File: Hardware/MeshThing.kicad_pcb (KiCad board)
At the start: 2 copper layers, 25.7 x 27.8 mm, 31 parts, among them IC1 ATMEGA2564/1284/644RFR2, SW1 RST, U1 CONN_MICROSD, U2 XBEE, U3 XBEE

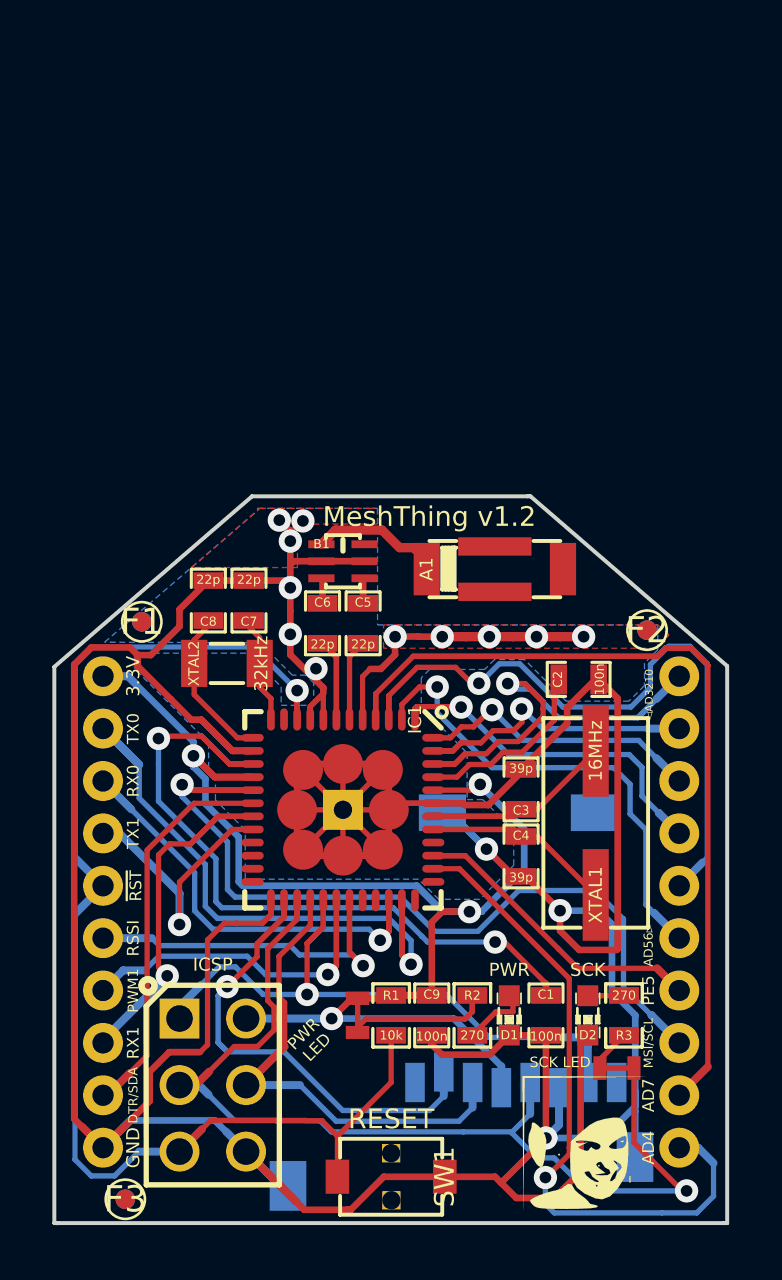
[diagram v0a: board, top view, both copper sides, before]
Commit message: Initial v2.0 commit.
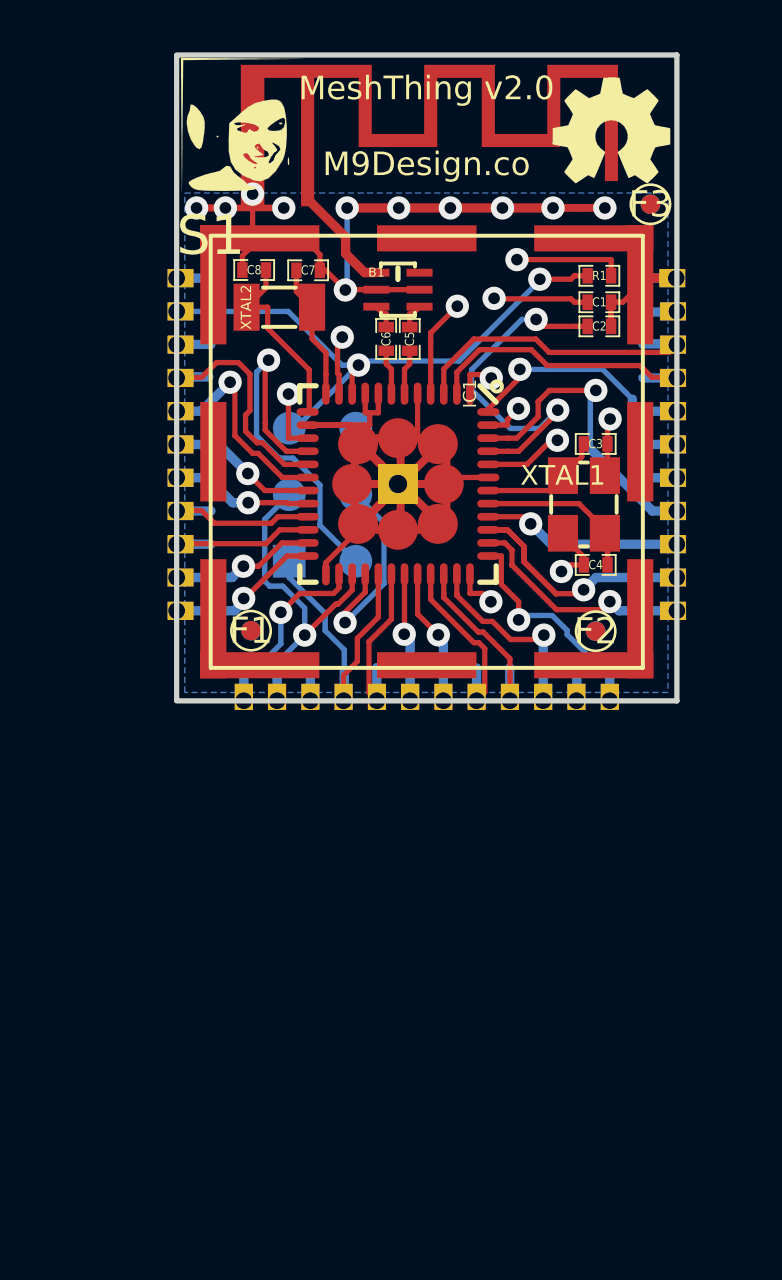
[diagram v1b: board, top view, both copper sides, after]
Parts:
- removed C9: 100n, _MT_SM0603_Capa
- removed D1, D2: LED, _MT_LED-0603
- removed the G*** at (155.9, 129.2)
- removed the G*** at (146.8, 108.7)
- removed H2: ICSP, _MT_pin_array_3x2
- removed R2, R3: 270, _MT_SM0603_Resistor
- removed SJ1, SJ2: SMTJPR, _MT_SMTJumper
- removed SW1: RST, _MT_TC007-TactileSwitch
- removed U1: CONN_MICROSD, _MT_microSD_3M_290805-A
- removed U2: XBEE, _MT_XBee_Board_STD_THPads
- removed U3: XBEE, _MT_XBee_Board_BackLablesOnly
- added G***: LOGO, _MT_OHW_LOGO:LOGO, F.Cu at (157.1, 90.5)
- added H1: ICSP, _MT_MC_Pretty:_MC_pin_pad_3x2, B.Cu at (146.0, 104.5)
- added P1: CONN34, _MT_MC_Pretty:_MC_CanFootprint-34Pin, F.Cu at (150.0, 100.0)
- added PrettyLady: PrettyLady, _MT_MC_Pretty:_MC_LOGO-PrettyLady, F.Cu at (142.9, 90.3)
- added S1: RFShield, _MT_MC_Pretty:_MT_MC_EMIShield-16.5x16.5, F.Cu at (150.0, 102.8)
- A1: value Antenna -> ANTENNA; footprint Johanson-2450AT42B100-PadsOnly -> _MT_MC_Pretty:_MT_IFA-2.4GHzPCBAntenna
- C1, C2, C5, C6, C7, C8: footprint _MT_SM0603_Capa -> SMD_Packages:SM0402_c
- C3, C4: value 39p -> 10p; footprint _MT_SM0603_Capa -> SMD_Packages:SM0402_c
- F1, F2, F3: value VAL** -> CONN_1; footprint _MT_Fiducial -> _MT_MC_Pretty:_MT_Fiducial
- R1: footprint _MT_SM0603_Resistor -> SMD_Packages:SM0402_r
- XTAL1: value 16MHz -> CRYSTAL_SMD-TSX3225; footprint _MT_CSM-3X-Crystal -> _MT_MC_Pretty:16MHz-3.2x2.5mm-TSX-3225
- XTAL2: footprint _MT_TF32D-32768-Crystal -> _MT_MC_Pretty:_MC_TF32D-32768-Crystal
- moved F3 43.0 mm to (158.5, 93.4)
- moved R1 29.3 mm to (156.6, 96.1), turned to 180 degrees
- moved C1 27.3 mm to (156.6, 97.1), turned to 0 degrees
- moved A1 16.9 mm to (150.0, 90.6)
- moved XTAL2 13.7 mm to (144.4, 97.3)
- moved C2 13.5 mm to (156.6, 98.0)
- moved C3 13.5 mm to (156.4, 102.5), turned to 0 degrees
- moved C7 12.8 mm to (145.5, 95.9), turned to 0 degrees
- moved C8 12.7 mm to (143.4, 95.9), turned to 180 degrees
- moved IC1 12.6 mm to (148.9, 104.0)
- moved XTAL1 12.2 mm to (156.0, 104.8), turned to 0 degrees
- moved C4 11.5 mm to (156.4, 107.1), turned to 180 degrees
- moved C6 11.1 mm to (148.4, 98.5)
- moved C5 11.0 mm to (149.3, 98.5)
- moved B1 10.6 mm to (148.9, 96.6)
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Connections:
- A1 pad 2: N-0000040 -> GND
- C3 pad 1: N-0000051 -> Net-(C3-Pad1)
- C4 pad 1: N-0000052 -> Net-(C4-Pad1)
- IC1 pad 11: N-0000049 -> PG1
- IC1 pad 21: N-0000048 -> PD4
- IC1 pad 22: N-0000047 -> PD5
- IC1 pad 23: N-0000046 -> PD6
- IC1 pad 24: N-0000044 -> PD7
- IC1 pad 32: N-0000021 -> PB6
- IC1 pad 33: N-0000045 -> PB7
- IC1 pad 36: N-0000022 -> PE2
- IC1 pad 37: N-0000020 -> PE3
- IC1 pad 40: N-0000050 -> PE7
- IC1 pad 41: N-0000052 -> Net-(C4-Pad1)
- IC1 pad 42: N-0000051 -> Net-(C3-Pad1)
- XTAL1 pad 1: N-0000052 -> Net-(C3-Pad1)
- XTAL1 pad 2: N-0000051 -> GND
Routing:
- net GND: track 226.8 -> 94.8 mm, vias 14 -> 13
- net PF7: track 45.6 -> 16.0 mm, vias 0 -> 1
- net Reset: track 49.1 -> 22.9 mm, vias 1 -> 2
- net SCK: track 39.6 -> 15.1 mm
- net SCL: track 33.1 -> 9.61 mm, vias 1 -> 0
- net PE4: track 25.6 -> 8.87 mm
- net TX0: track 24.8 -> 9.87 mm
- net PF6: track 26.3 -> 12.0 mm, vias 1 -> 0
- net PE7: track 0.00 -> 13.5 mm, vias 0 -> 1
- net MISO: track 25.1 -> 11.6 mm, vias 1 -> 0
- net Net-(C1-Pad1): track 28.0 -> 15.5 mm
- net PG1: track 0.00 -> 11.0 mm, vias 0 -> 1
- net N-0000052: track 10.7 -> 0.00 mm
- net N-0000051: track 10.7 -> 0.00 mm
- net RX0: track 17.3 -> 7.22 mm, vias 1 -> 0
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- added copper zone on Inner1.Cu, net +3.3V
- added copper zone on Inner2.Cu, net GND
- removed copper zone on F.Cu, net GND
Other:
- board size 25.7 x 27.8 mm -> 19.1 x 24.7 mm
- copper layers 2 -> 4
- net class 10mil added: clearance 0.2032, trace_width 0.254, via_dia 0.889, via_drill 0.635
- net class Default: trace_width 0.254 -> 0.2032
- board text added: "MeshThing v2.0 M9Design.co"
- board text added: "MeshThing v2.0 © M9Design.co 2013 Designed by Robert Powers"
- board text added: "OpenHardware Under TAPR OHL tapr.org/OHL"
- board text removed: "MeshThing v1.2"
- board text removed: "PWR"
- board text removed: "PWR LED"
- board text removed: "RESET"
- board text removed: "SCK"
- board text removed: "SCK LED"
- board text removed: "©BobPowers 2013 OpenHardware Under TAPR OHL tapr.org/OHL"
